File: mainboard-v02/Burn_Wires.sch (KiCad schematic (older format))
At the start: 41 parts, among them Q2 2N5088, Q3 2N5088, Q4 IRLML2803, Q5 IRLML2803, Q6 IRLML2803, Q7 IRLML2803, Q8 IRLML2803, U16 PE014006, U17 PE014006, U18 NDS8434, U19 NDS8434, U20 NDS8434, U21 NDS8434, U22 NDS8434

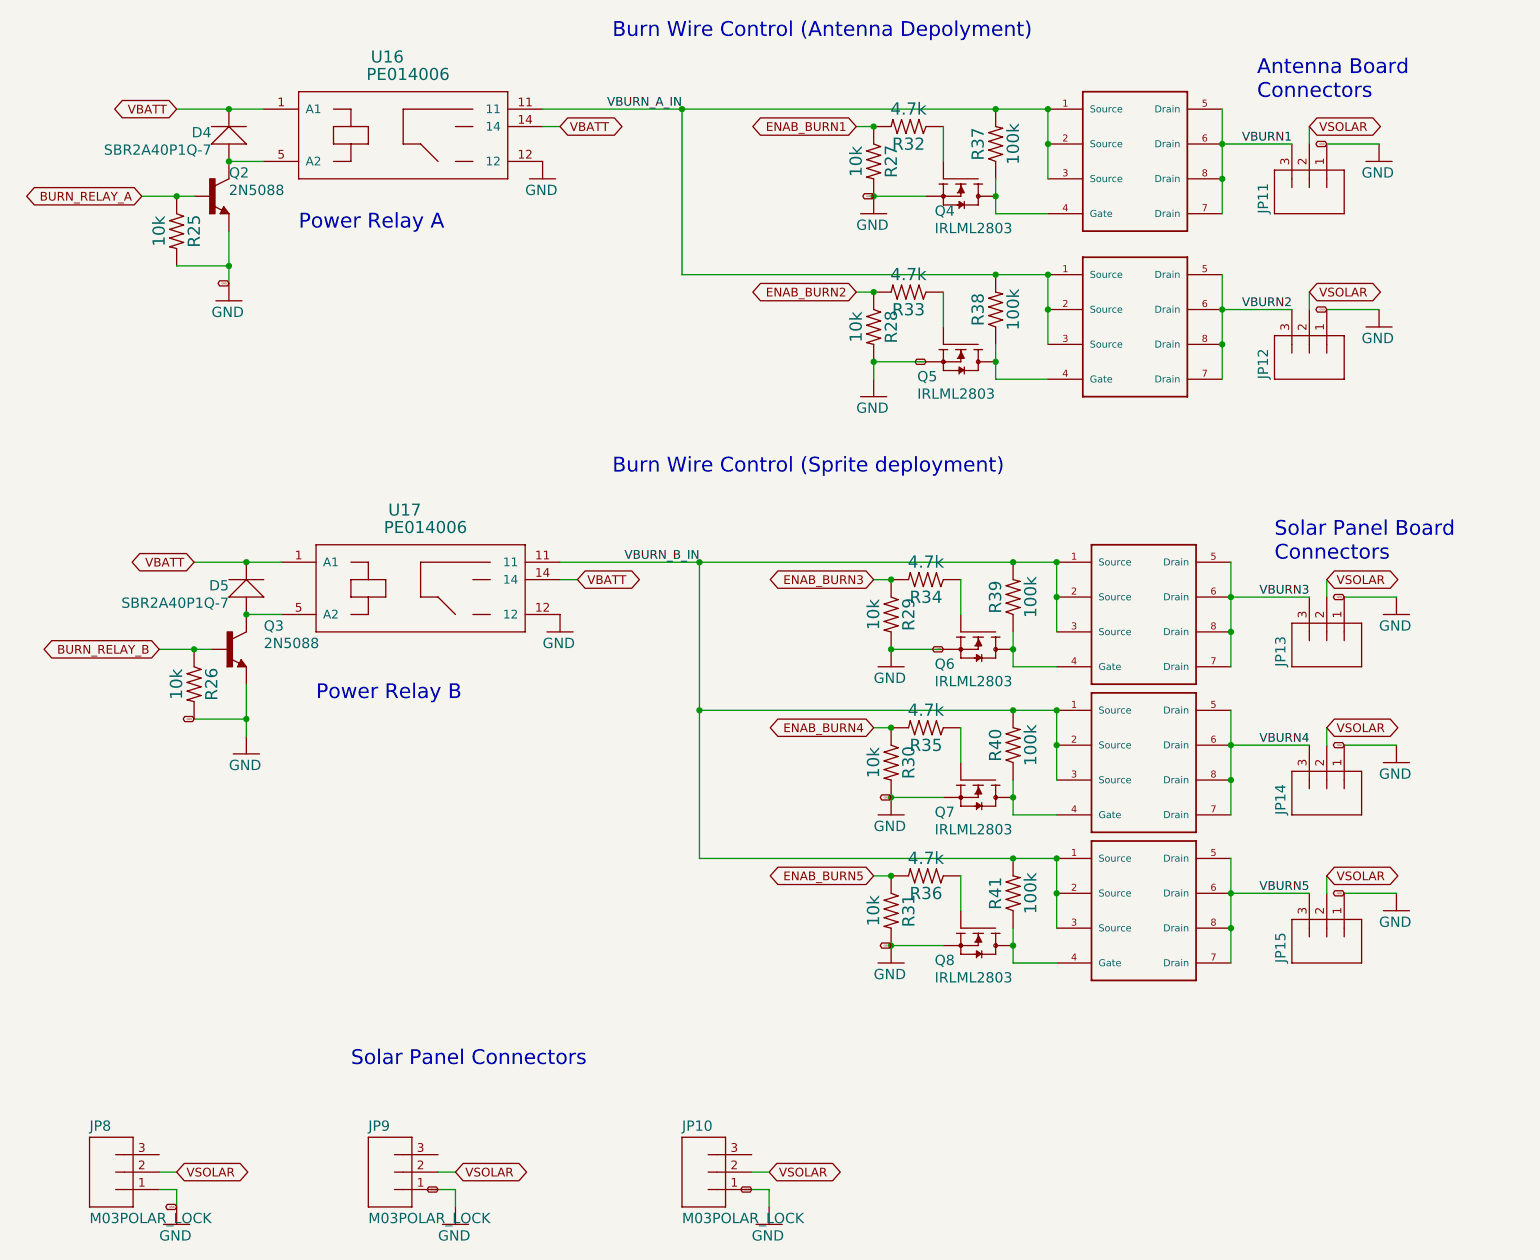
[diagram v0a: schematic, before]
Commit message: fixing bold font and adding schematic pdf of v02
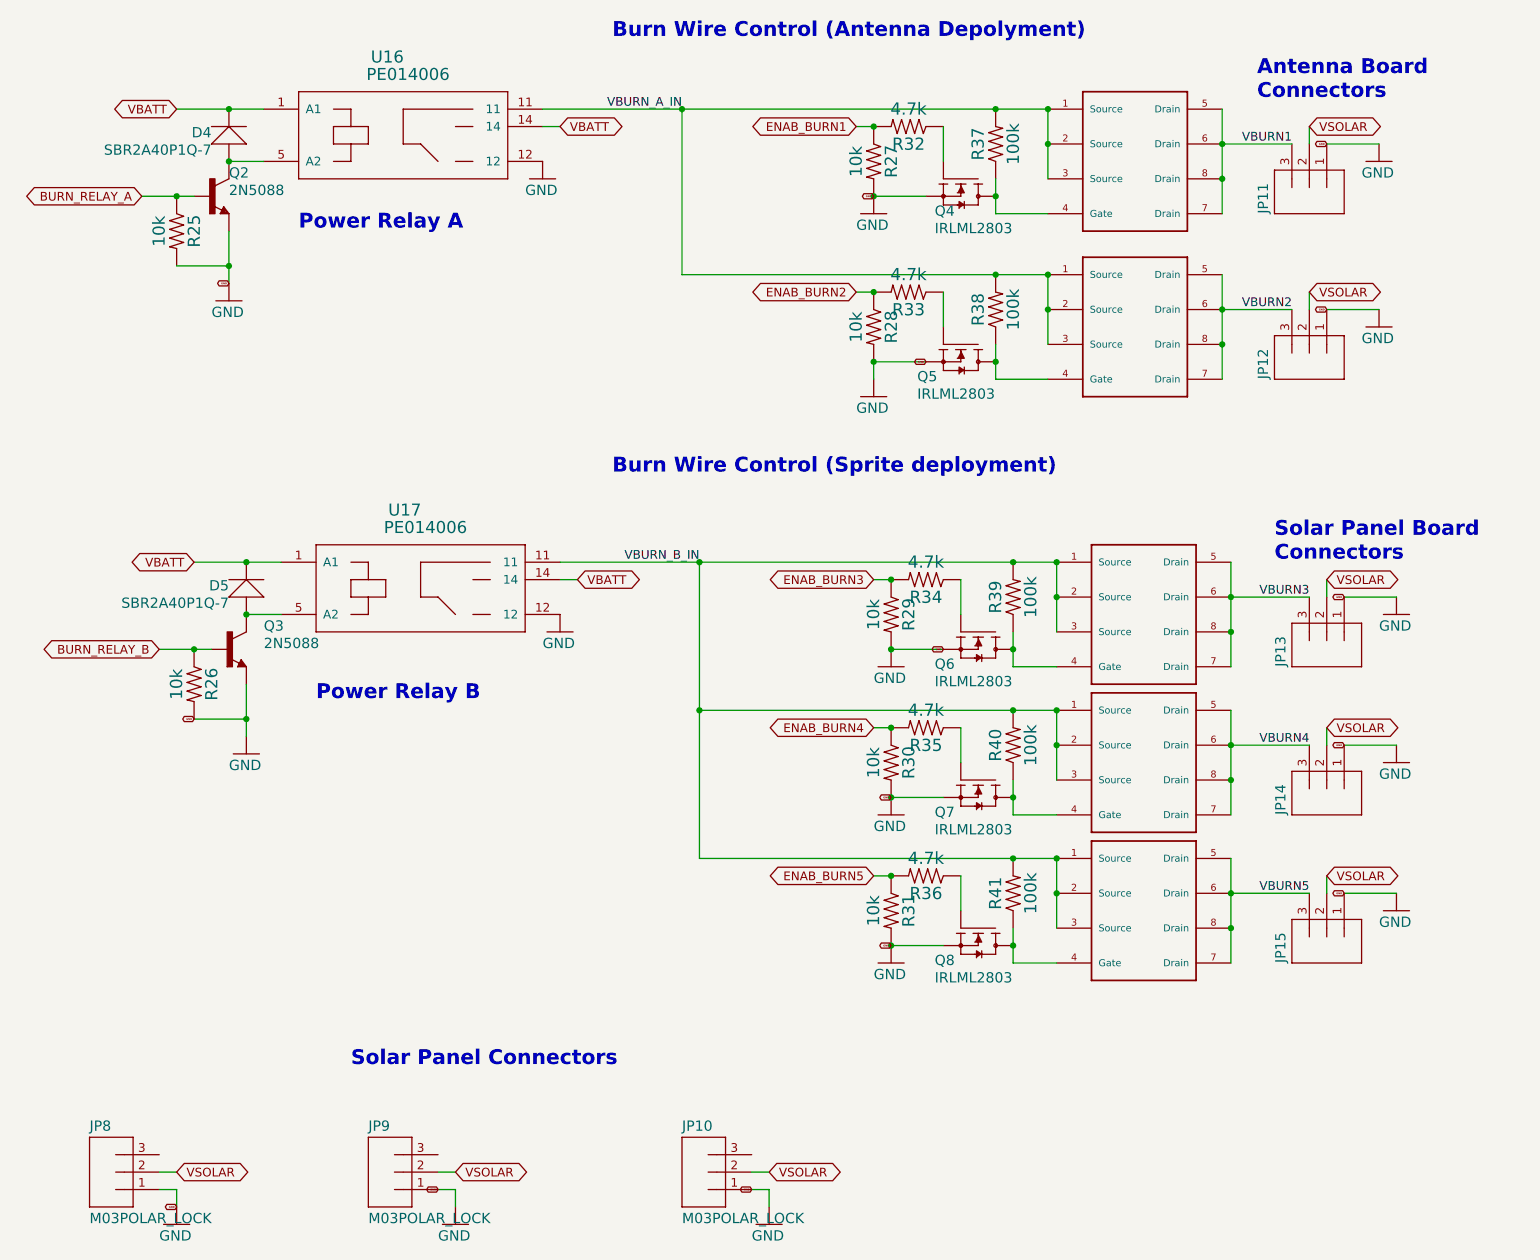
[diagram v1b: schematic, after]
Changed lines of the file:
@@
 EESchema Schematic File Version 4
-LIBS:mainboard
 EELAYER 29 0
 EELAYER END
@@
 	6000 1700 6300 1700
 Connection ~ 6000 1700
-Text GLabel 6000 1700 0    10   BiDi ~ 0
+Text GLabel 6000 1700 0    10   BiDi ~ 2
 GND
 Wire Wire Line
@@
 	6000 2650 6000 2750
 Connection ~ 6000 2650
-Text GLabel 6300 2650 0    10   BiDi ~ 0
+Text GLabel 6300 2650 0    10   BiDi ~ 2
 GND
 Wire Wire Line
 	6400 4300 6100 4300
 Connection ~ 6100 4300
-Text GLabel 6400 4300 0    10   BiDi ~ 0
+Text GLabel 6400 4300 0    10   BiDi ~ 2
 GND
 Wire Wire Line
 	6100 5150 6400 5150
 Connection ~ 6100 5150
-Text GLabel 6100 5150 0    10   BiDi ~ 0
+Text GLabel 6100 5150 0    10   BiDi ~ 2
 GND
 Wire Wire Line
 	6100 6000 6400 6000
 Connection ~ 6100 6000
-Text GLabel 6100 6000 0    10   BiDi ~ 0
+Text GLabel 6100 6000 0    10   BiDi ~ 2
 GND
 Wire Wire Line
 	8600 2350 8900 2350
-Text GLabel 8600 2350 0    10   BiDi ~ 0
+Text GLabel 8600 2350 0    10   BiDi ~ 2
 GND
 Wire Wire Line
 	8700 4000 9000 4000
-Text GLabel 8700 4000 0    10   BiDi ~ 0
+Text GLabel 8700 4000 0    10   BiDi ~ 2
 GND
 Wire Wire Line
@@
 Wire Wire Line
 	5400 7400 5400 7500
-Text GLabel 5300 7400 0    10   BiDi ~ 0
+Text GLabel 5300 7400 0    10   BiDi ~ 2
 GND
 Wire Wire Line
@@
 Wire Wire Line
 	2000 7400 1900 7400
-Text GLabel 2000 7500 0    10   BiDi ~ 0
+Text GLabel 2000 7500 0    10   BiDi ~ 2
 GND
 Wire Wire Line
@@
 Wire Wire Line
 	3600 7400 3600 7500
-Text GLabel 3500 7400 0    10   BiDi ~ 0
+Text GLabel 3500 7400 0    10   BiDi ~ 2
 GND
 Wire Wire Line
 	8600 1400 8900 1400
-Text GLabel 8600 1400 0    10   BiDi ~ 0
+Text GLabel 8600 1400 0    10   BiDi ~ 2
 GND
 Wire Wire Line
 	8700 4850 9000 4850
-Text GLabel 8700 4850 0    10   BiDi ~ 0
+Text GLabel 8700 4850 0    10   BiDi ~ 2
 GND
 Wire Wire Line
 	8700 5700 9000 5700
-Text GLabel 8700 5700 0    10   BiDi ~ 0
+Text GLabel 8700 5700 0    10   BiDi ~ 2
 GND
 Wire Wire Line
@@
 	2000 2100 2300 2100
 Connection ~ 2300 2100
-Text GLabel 2300 2200 0    10   BiDi ~ 0
+Text GLabel 2300 2200 0    10   BiDi ~ 2
 GND
 Wire Wire Line
@@
 	2400 4500 2400 4700
 Connection ~ 2400 4700
-Text GLabel 2100 4700 0    10   BiDi ~ 0
+Text GLabel 2100 4700 0    10   BiDi ~ 2
 GND
 Text Label 8500 4000 2    50   ~ 0
@@
 	0    -1   -1   0
 $EndComp
-Text Notes 2700 1900 0    85   ~ 0
+Text Notes 2700 1900 0    85   ~ 17
 Power Relay A
-Text Notes 4500 800  0    85   ~ 0
+Text Notes 4500 800  0    85   ~ 17
 Burn Wire Control (Antenna Depolyment)
-Text Notes 4500 3300 0    85   ~ 0
+Text Notes 4500 3300 0    85   ~ 17
 Burn Wire Control (Sprite deployment)
-Text Notes 2800 4600 0    85   ~ 0
+Text Notes 2800 4600 0    85   ~ 17
 Power Relay B
-Text Notes 8200 1150 0    85   ~ 0
+Text Notes 8200 1150 0    85   ~ 17
 Antenna Board\nConnectors
-Text Notes 8300 3800 0    85   ~ 0
+Text Notes 8300 3800 0    85   ~ 17
 Solar Panel Board\nConnectors
-Text Notes 3000 6700 0    85   ~ 0
+Text Notes 3000 6700 0    85   ~ 17
 Solar Panel Connectors
 Wire Wire Line
